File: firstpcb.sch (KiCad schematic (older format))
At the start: 24 parts, among them SW1 SW_Push, U1 ATmega32U4-AU, Y1 16MHz

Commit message: footprint
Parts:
- SW1: footprint (none) -> random-keyboard-parts:SKQG-1155865
- USB1: footprint (none) -> random-keyboard-parts:Molex-0548190589
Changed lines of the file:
@@
 F 0 "SW1" H 3900 2185 50  0000 C CNN
 F 1 "SW_Push" H 3900 2094 50  0000 C CNN
-F 2 "" H 3900 2100 50  0001 C CNN
+F 2 "random-keyboard-parts:SKQG-1155865" H 3900 2100 50  0001 C CNN
 F 3 "~" H 3900 2100 50  0001 C CNN
 	1    3900 1900
@@
 F 0 "USB1" V 7287 2017 60  0000 C CNN
 F 1 "Molex-0548190589" V 7181 2017 60  0000 C CNN
-F 2 "" H 6750 2050 60  0001 C CNN
+F 2 "random-keyboard-parts:Molex-0548190589" H 6750 2050 60  0001 C CNN
 F 3 "" H 6750 2050 60  0001 C CNN
 	1    6750 2050

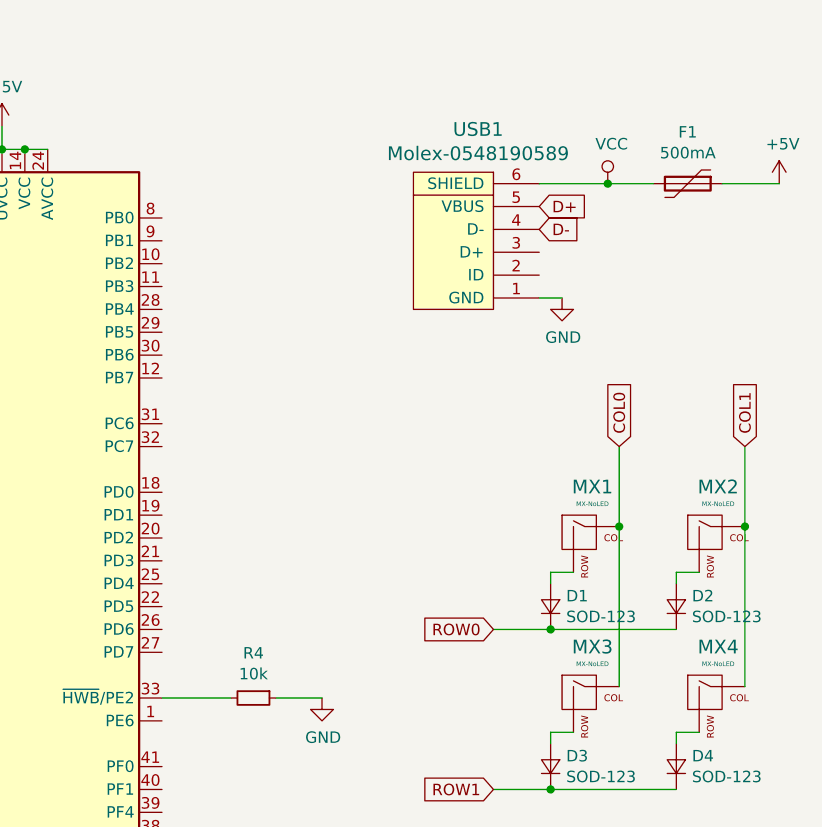
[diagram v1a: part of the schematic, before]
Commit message: 0
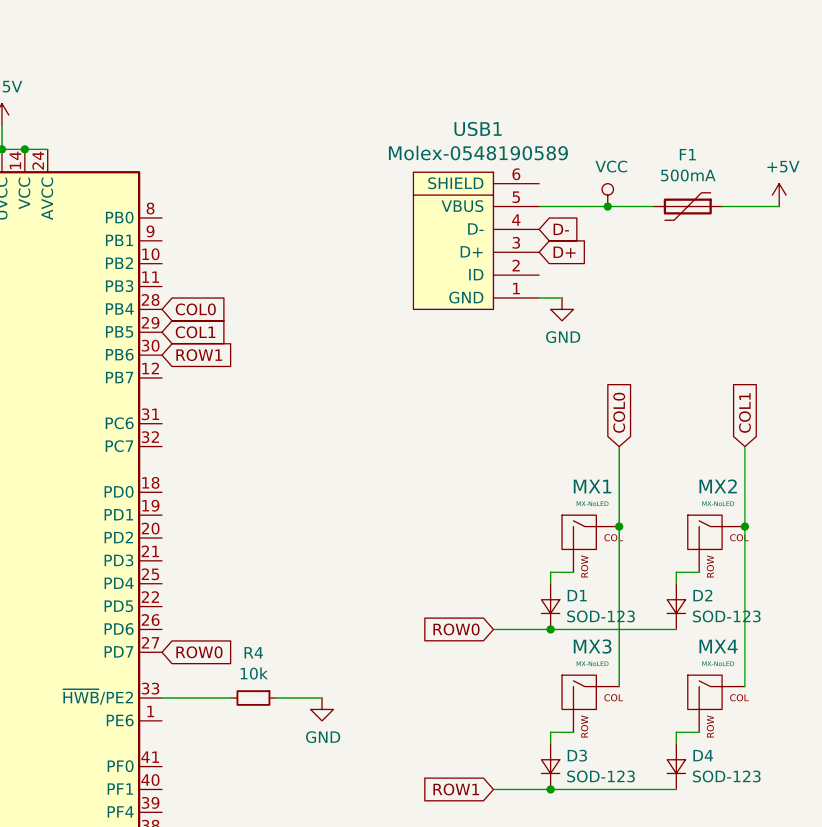
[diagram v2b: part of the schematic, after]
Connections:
- net COL0: now also U1.28 (PB4)
- net COL1: now also U1.29 (PB5)
- net D+: now also USB1.3 (D+); no longer USB1.5 (VBUS)
- net ROW0: now also U1.27 (PD7)
- net ROW1: now also U1.30 (PB6)
- net VCC: now also USB1.5 (VBUS); no longer USB1.6 (SHIELD)
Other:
- moved on the sheet: F1
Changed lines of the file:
@@
 L power:VCC #PWR0111
 U 1 1 636C0166
-P 7350 1750
-F 0 "#PWR0111" H 7350 1600 50  0001 C CNN
-F 1 "VCC" H 7367 1923 50  0000 C CNN
-F 2 "" H 7350 1750 50  0001 C CNN
-F 3 "" H 7350 1750 50  0001 C CNN
-	1    7350 1750
+P 7350 1850
+F 0 "#PWR0111" H 7350 1700 50  0001 C CNN
+F 1 "VCC" H 7367 2023 50  0000 C CNN
+F 2 "" H 7350 1850 50  0001 C CNN
+F 3 "" H 7350 1850 50  0001 C CNN
+	1    7350 1850
 	1    0    0    -1
 $EndComp
@@
 L Device:Polyfuse F1
 U 1 1 636C3A9A
-P 7700 1750
-F 0 "F1" V 7475 1750 50  0000 C CNN
-F 1 "500mA" V 7566 1750 50  0000 C CNN
-F 2 "Fuse:Fuse_1206_3216Metric" H 7750 1550 50  0001 L CNN
-F 3 "~" H 7700 1750 50  0001 C CNN
-	1    7700 1750
+P 7700 1850
+F 0 "F1" V 7475 1850 50  0000 C CNN
+F 1 "500mA" V 7566 1850 50  0000 C CNN
+F 2 "Fuse:Fuse_1206_3216Metric" H 7750 1650 50  0001 L CNN
+F 3 "~" H 7700 1850 50  0001 C CNN
+	1    7700 1850
 	0    1    1    0
 $EndComp
@@
 L power:+5V #PWR0112
 U 1 1 636C5D2B
-P 8100 1750
-F 0 "#PWR0112" H 8100 1600 50  0001 C CNN
-F 1 "+5V" H 8115 1923 50  0000 C CNN
-F 2 "" H 8100 1750 50  0001 C CNN
-F 3 "" H 8100 1750 50  0001 C CNN
-	1    8100 1750
+P 8100 1850
+F 0 "#PWR0112" H 8100 1700 50  0001 C CNN
+F 1 "+5V" H 8115 2023 50  0000 C CNN
+F 2 "" H 8100 1850 50  0001 C CNN
+F 3 "" H 8100 1850 50  0001 C CNN
+	1    8100 1850
 	1    0    0    -1
 $EndComp
 Wire Wire Line
-	7050 1750 7350 1750
+	7050 1850 7350 1850
 Wire Wire Line
-	7850 1750 8100 1750
-Connection ~ 7350 1750
+	7850 1850 8100 1850
+Connection ~ 7350 1850
 Wire Wire Line
-	7350 1750 7550 1750
+	7350 1850 7550 1850
 $Comp
 L power:GND #PWR0113
@@
 	1    0    0    -1
 $EndComp
+Text GLabel 7050 2050 2    50   Input ~ 0
+D+
 Text GLabel 7050 1950 2    50   Input ~ 0
 D-
-Text GLabel 7050 1850 2    50   Input ~ 0
-D+
 Wire Wire Line
 	7050 2250 7150 2250
@@
 Text GLabel 6850 4400 0    50   Input ~ 0
 ROW1
+Text GLabel 5400 2400 2    50   Input ~ 0
+COL1
+Text GLabel 5400 2300 2    50   Input ~ 0
+COL0
+Text GLabel 5400 3800 2    50   Input ~ 0
+ROW0
+Text GLabel 5400 2500 2    50   Input ~ 0
+ROW1
 $EndSCHEMATC
